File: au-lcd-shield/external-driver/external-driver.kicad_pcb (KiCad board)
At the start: 2 copper layers, 65 x 45 mm, 8 parts, among them IC2 DSLVDS1047PWR, J1 Power, J2 Backlight, J4 Conn_02x09_Odd_Even, U1 78M05

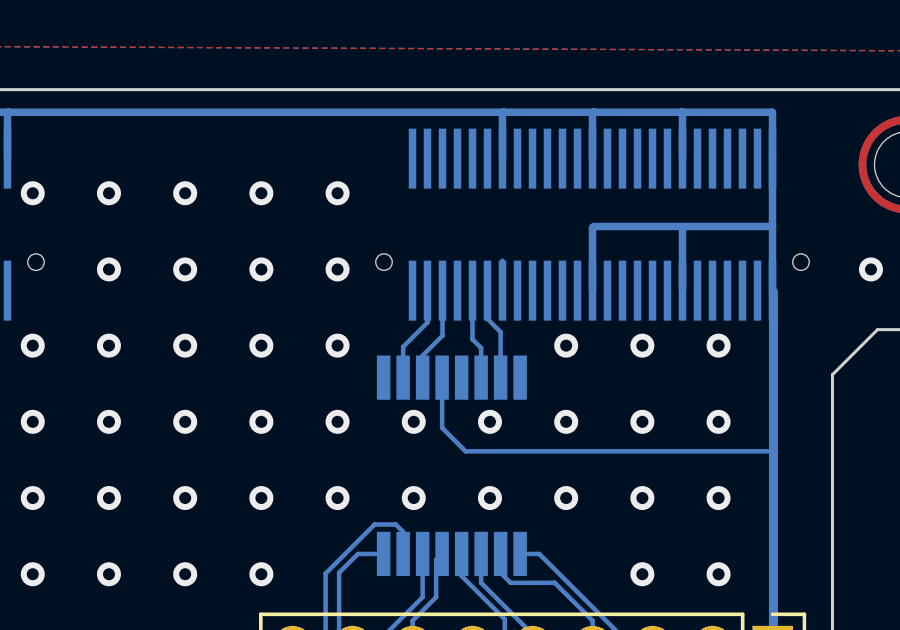
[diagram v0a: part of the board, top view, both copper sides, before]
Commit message: fix pins WIP
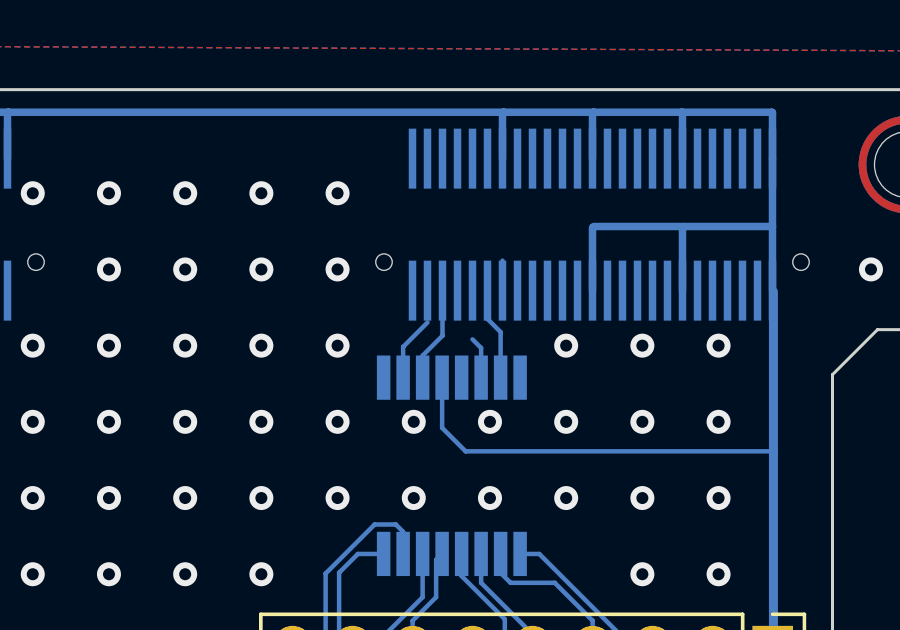
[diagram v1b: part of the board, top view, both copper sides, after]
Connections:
- B1 pad B_12: unconnected-(B1B-F4-PadB_12) -> TX1_B_IN
- B1 pad B_2: TXCLK_B_IN -> unconnected-(B1B-D1-PadB_2)
- B1 pad B_5: TX1_B_IN -> unconnected-(B1B-A2-PadB_5)
- B1 pad B_9: unconnected-(B1B-F2-PadB_9) -> TXCLK_B_IN
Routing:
- net TX1_B_IN: track 3.02 -> 1.40 mm
- net TXCLK_B_IN: track 3.24 -> 2.17 mm
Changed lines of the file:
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@@
   (net 5 "TX2_B_IN")
   (net 6 "TXCLK_B_IN")
-  (net 7 "unconnected-(B1B-F2-PadB_9)")
+  (net 7 "unconnected-(B1B-D1-PadB_2)")
   (net 8 "unconnected-(B1B-E1-PadB_8)")
   (net 9 "TXCLK_P")
@@
   (net 41 "unconnected-(B1A-T10-PadA_49)")
   (net 42 "unconnected-(B1B-F3-PadB_11)")
-  (net 43 "unconnected-(B1B-F4-PadB_12)")
+  (net 43 "unconnected-(B1B-A2-PadB_5)")
   (net 44 "unconnected-(B1B-A3-PadB_14)")
   (net 45 "unconnected-(B1B-B4-PadB_15)")
@@
       (net 134 "+5V") (pinfunction "5V") (pintype "passive") (solder_mask_margin 0.102))
     (pad "B_2" smd rect locked (at 46.5 -38.3 90) (size 2 0.25) (layers "B.Cu" "B.Paste" "B.Mask")
-      (net 6 "TXCLK_B_IN") (pinfunction "D1") (pintype "passive") (solder_mask_margin 0.102))
+      (net 7 "unconnected-(B1B-D1-PadB_2)") (pinfunction "D1") (pintype "passive") (solder_mask_margin 0.102))
     (pad "B_3" smd rect locked (at 47 -38.3 90) (size 2 0.25) (layers "B.Cu" "B.Paste" "B.Mask")
       (net 5 "TX2_B_IN") (pinfunction "E2") (pintype "passive") (solder_mask_margin 0.102))
@@
       (net 1 "GND") (pinfunction "GND") (pintype "passive") (solder_mask_margin 0.102))
     (pad "B_5" smd rect locked (at 48 -38.3 90) (size 2 0.25) (layers "B.Cu" "B.Paste" "B.Mask")
-      (net 4 "TX1_B_IN") (pinfunction "A2") (pintype "passive") (solder_mask_margin 0.102))
+      (net 43 "unconnected-(B1B-A2-PadB_5)") (pinfunction "A2") (pintype "passive") (solder_mask_margin 0.102))
     (pad "B_6" smd rect locked (at 48.5 -38.3 90) (size 2 0.25) (layers "B.Cu" "B.Paste" "B.Mask")
-      (net 3 "TX0_B_IN") (pinfunction "E2") (pintype "passive") (solder_mask_margin 0.102))
+      (net 3 "TX0_B_IN") (pinfunction "B2") (pintype "passive") (solder_mask_margin 0.102))
     (pad "B_7" smd rect locked (at 49 -38.3 90) (size 2 0.25) (layers "B.Cu" "B.Paste" "B.Mask")
       (net 2 "+3.3V") (pinfunction "3V3") (pintype "passive") (solder_mask_margin 0.102))
@@
       (net 8 "unconnected-(B1B-E1-PadB_8)") (pinfunction "E1") (pintype "passive") (solder_mask_margin 0.102))
     (pad "B_9" smd rect locked (at 50 -38.3 90) (size 2 0.25) (layers "B.Cu" "B.Paste" "B.Mask")
-      (net 7 "unconnected-(B1B-F2-PadB_9)") (pinfunction "F2") (pintype "passive") (solder_mask_margin 0.102))
+      (net 6 "TXCLK_B_IN") (pinfunction "F2") (pintype "passive") (solder_mask_margin 0.102))
     (pad "B_10" smd rect locked (at 50.5 -38.3 90) (size 2 0.25) (layers "B.Cu" "B.Paste" "B.Mask")
       (net 1 "GND") (pinfunction "GND") (pintype "passive") (solder_mask_margin 0.102))
@@
       (net 42 "unconnected-(B1B-F3-PadB_11)") (pinfunction "F3") (pintype "passive") (solder_mask_margin 0.102))
     (pad "B_12" smd rect locked (at 51.5 -38.3 90) (size 2 0.25) (layers "B.Cu" "B.Paste" "B.Mask")
-      (net 43 "unconnected-(B1B-F4-PadB_12)") (pinfunction "F4") (pintype "passive") (solder_mask_margin 0.102))
+      (net 4 "TX1_B_IN") (pinfunction "F4") (pintype "passive") (solder_mask_margin 0.102))
     (pad "B_13" smd rect locked (at 52 -38.3 90) (size 2 0.25) (layers "B.Cu" "B.Paste" "B.Mask")
       (net 2 "+3.3V") (pinfunction "3V3") (pintype "passive") (solder_mask_margin 0.102))
@@
       (stroke (width 0.1) (type solid)) (layer "B.Fab"))
     (pad "1" smd rect (at -2.938 2.275 180) (size 0.45 1.475) (layers "B.Cu" "B.Paste" "B.Mask")
-      (net 136 "unconnected-(IC2-EN_1-Pad1)") (pinfunction "EN_1") (pintype "passive"))
+      (net 136 "unconnected-(IC2-EN_1-Pad1)") (pinfunction "EN_1") (pintype "passive+no_connect"))
     (pad "2" smd rect (at -2.938 1.625 180) (size 0.45 1.475) (layers "B.Cu" "B.Paste" "B.Mask")
       (net 6 "TXCLK_B_IN") (pinfunction "DIN1") (pintype "passive"))
@@
       (net 3 "TX0_B_IN") (pinfunction "DIN4") (pintype "passive"))
     (pad "8" smd rect (at -2.938 -2.275 180) (size 0.45 1.475) (layers "B.Cu" "B.Paste" "B.Mask")
-      (net 137 "unconnected-(IC2-EN_2-Pad8)") (pinfunction "EN_2") (pintype "passive"))
+      (net 137 "unconnected-(IC2-EN_2-Pad8)") (pinfunction "EN_2") (pintype "passive+no_connect"))
     (pad "9" smd rect (at 2.938 -2.275 180) (size 0.45 1.475) (layers "B.Cu" "B.Paste" "B.Mask")
       (net 17 "TX0_N") (pinfunction "DOUT4-") (pintype "passive"))
@@
   (segment (start 160.375 87.1304) (end 160.375 85.610698) (width 0.15) (layer "B.Cu") (net 3))
   (segment (start 159.725 87.1304) (end 159.725 86.1412) (width 0.15) (layer "B.Cu") (net 4))
-  (segment (start 159.4375 85.8537) (end 159.4375 84.23) (width 0.15) (layer "B.Cu") (net 4))
   (segment (start 159.725 86.1412) (end 159.4375 85.8537) (width 0.15) (layer "B.Cu") (net 4))
   (segment (start 157.775 86.3952) (end 158.4375 85.7327) (width 0.15) (layer "B.Cu") (net 5))
   (segment (start 157.775 87.1304) (end 157.775 86.3952) (width 0.15) (layer "B.Cu") (net 5))
   (segment (start 158.4375 85.7327) (end 158.4375 84.23) (width 0.15) (layer "B.Cu") (net 5))
-  (segment (start 157.9375 85.2929) (end 157.9375 84.23) (width 0.15) (layer "B.Cu") (net 6))
   (segment (start 157.125 86.1054) (end 157.9375 85.2929) (width 0.15) (layer "B.Cu") (net 6))
   (segment (start 157.125 87.1304) (end 157.125 86.1054) (width 0.15) (layer "B.Cu") (net 6))
